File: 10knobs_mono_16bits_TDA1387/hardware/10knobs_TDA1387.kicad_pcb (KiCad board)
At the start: 2 copper layers, 59 parts, among them J1 Prog - GND, SW1 SW_SPDT, U1 TDA1387, U2 BluePill_STM32F103C_breadboar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, U3 6N138, U4 TL072, U5 TL072

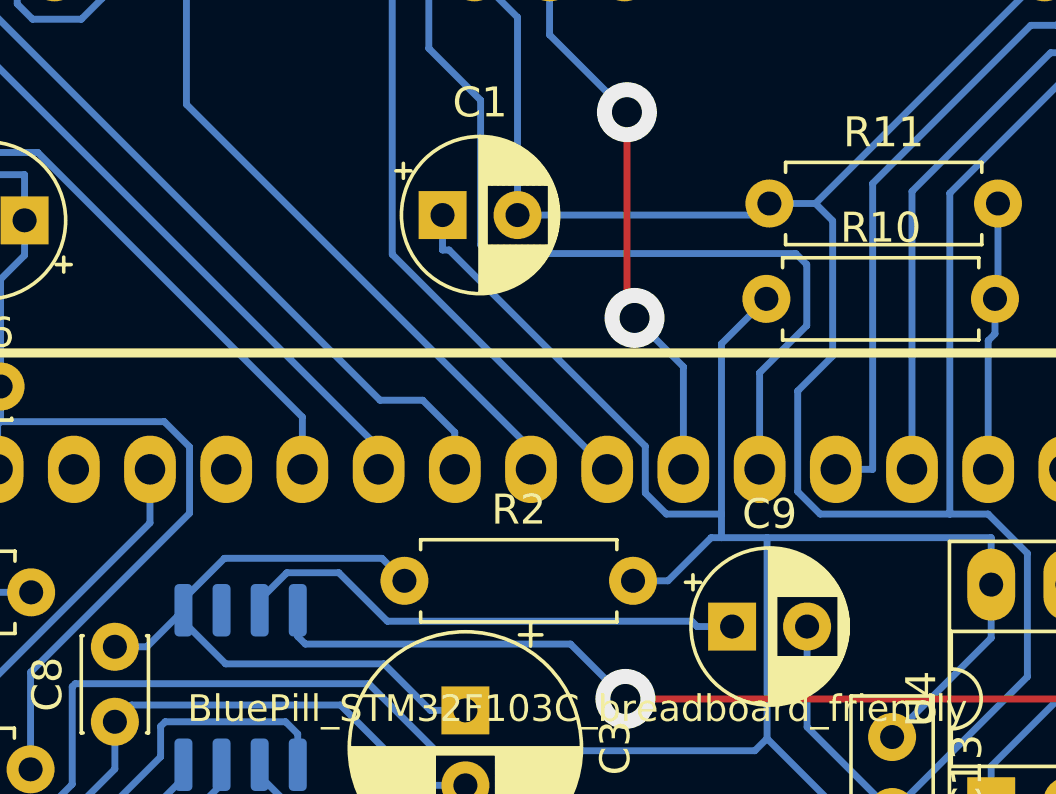
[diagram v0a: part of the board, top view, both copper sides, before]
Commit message: Updated PCB
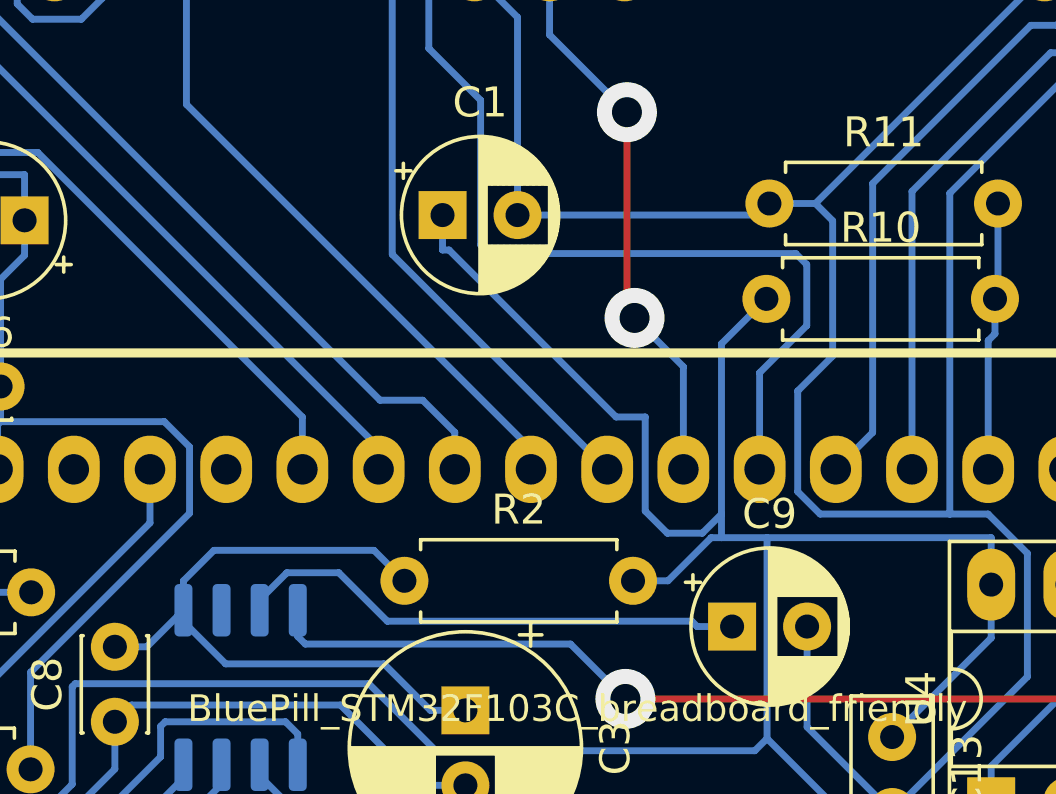
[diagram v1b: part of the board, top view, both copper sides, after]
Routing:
- net batt+: track 216.0 -> 217.5 mm
- net Net-(RV6-Pad2): track 21.9 -> 21.2 mm
- net Net-(C3-Pad1): track 22.3 -> 22.9 mm
